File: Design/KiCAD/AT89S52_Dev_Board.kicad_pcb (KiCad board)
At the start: 2 copper layers, 120 x 75 mm, 35 parts, among them J1 Jack-DC, J10 ISP, J11 LCD Port, J2 12V AC, J3 VCC_12V, J4 VCC_5V, J5 Port 3, J6 Port 1, J7 Port 2, J8 Port 0, J9 Serial Port, SW1 Reset, SW2 SW_Push, U1 L7812, U2 L7805, U3 AT89S52, U4 MAX232, Y1 Crystal

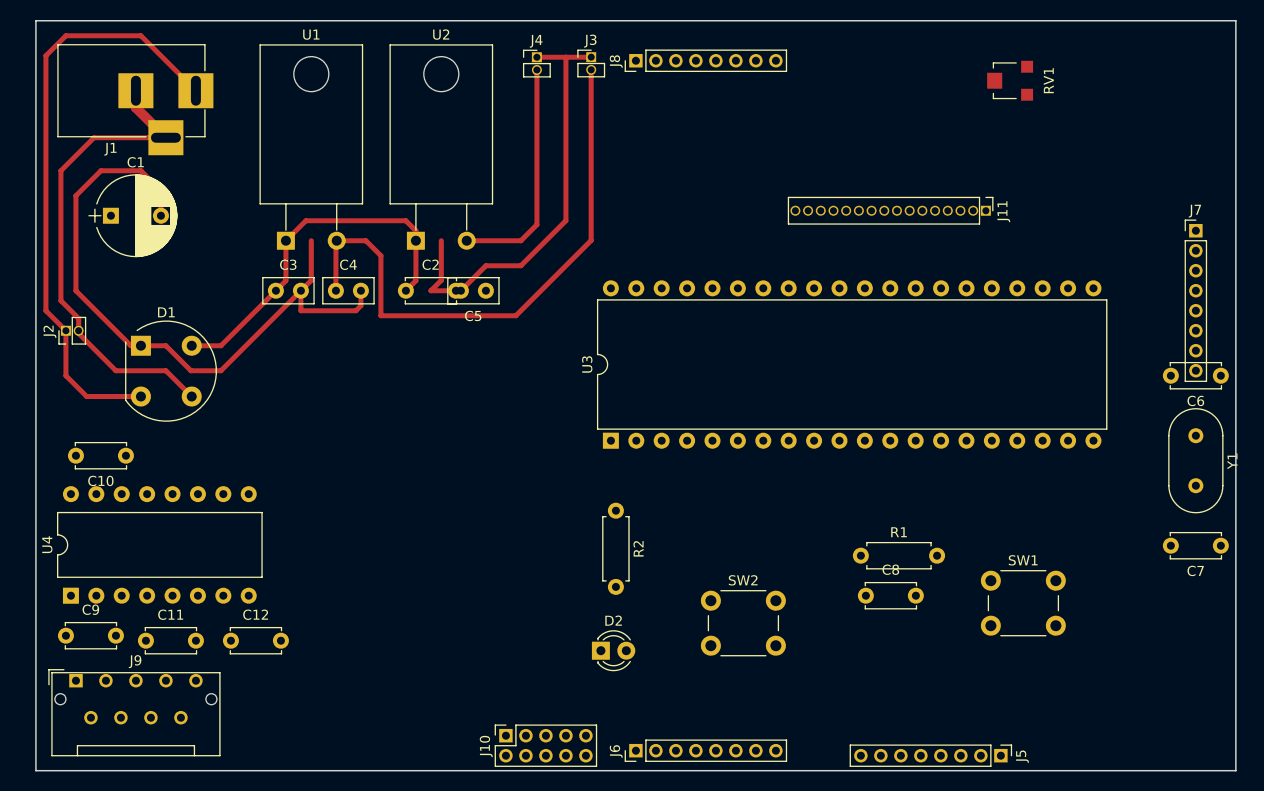
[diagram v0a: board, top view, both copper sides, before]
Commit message: modified
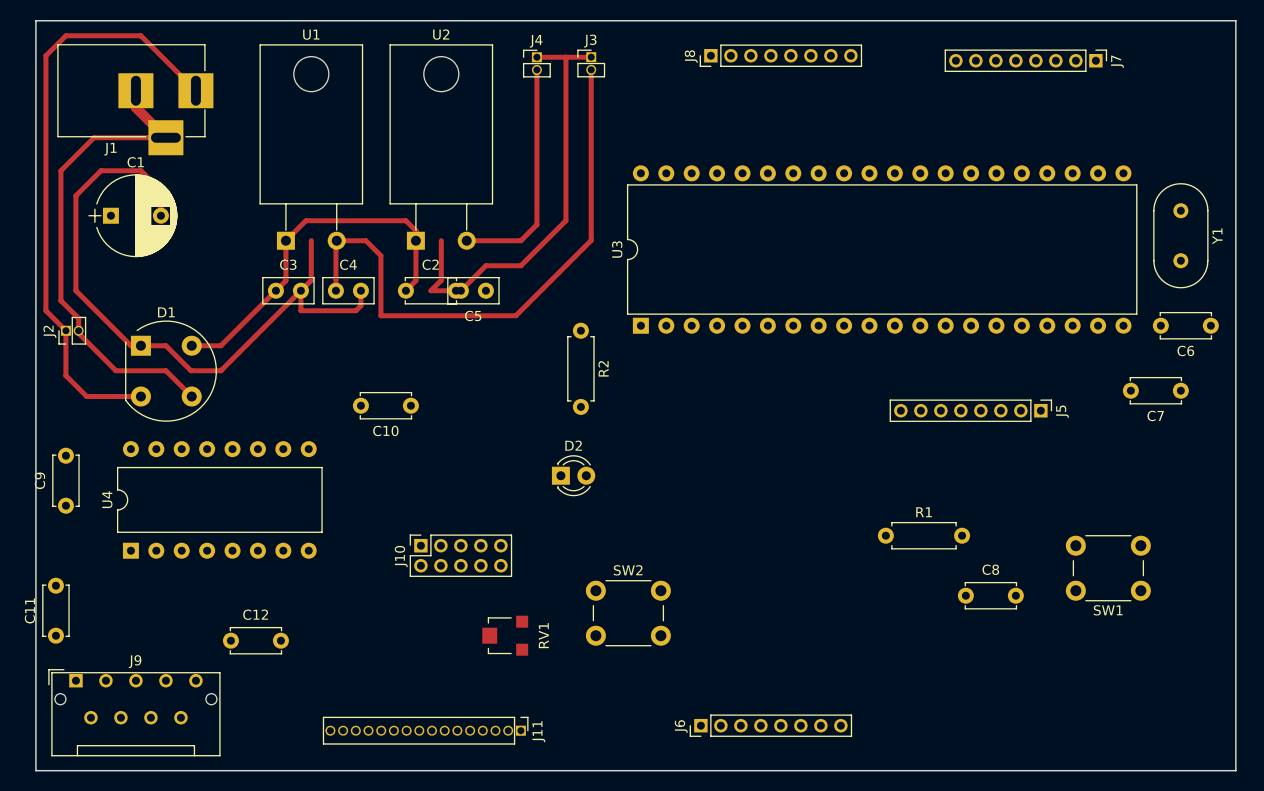
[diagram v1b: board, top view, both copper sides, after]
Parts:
- moved RV1 75.0 mm to (72.5, 77.5)
- moved J11 69.8 mm to (74.0, 87.0)
- moved J5 34.7 mm to (126.0, 55.0)
- moved C10 28.9 mm to (63.0, 54.5)
- moved Y1 22.5 mm to (140.0, 35.0)
- moved J10 20.8 mm to (64.0, 68.5)
- moved J7 19.7 mm to (131.5, 20.0), turned to 270 degrees
- moved R2 18.3 mm to (80.0, 47.0)
- moved D2 18.0 mm to (78.0, 61.5)
- moved C7 16.0 mm to (140.0, 53.0)
- moved SW1 15.0 mm to (136.0, 73.0), turned to 180 degrees
- moved C9 13.0 mm to (28.5, 64.5), turned to 90 degrees
- moved U3 11.9 mm to (86.0, 46.5)
- moved SW2 11.5 mm to (81.5, 73.0)
- moved C8 10.0 mm to (118.5, 73.5)
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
